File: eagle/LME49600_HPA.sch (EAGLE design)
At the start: 23 parts, among them IC1 OPA2134P, P1 POLYSWITCH, P2 POLYSWITCH

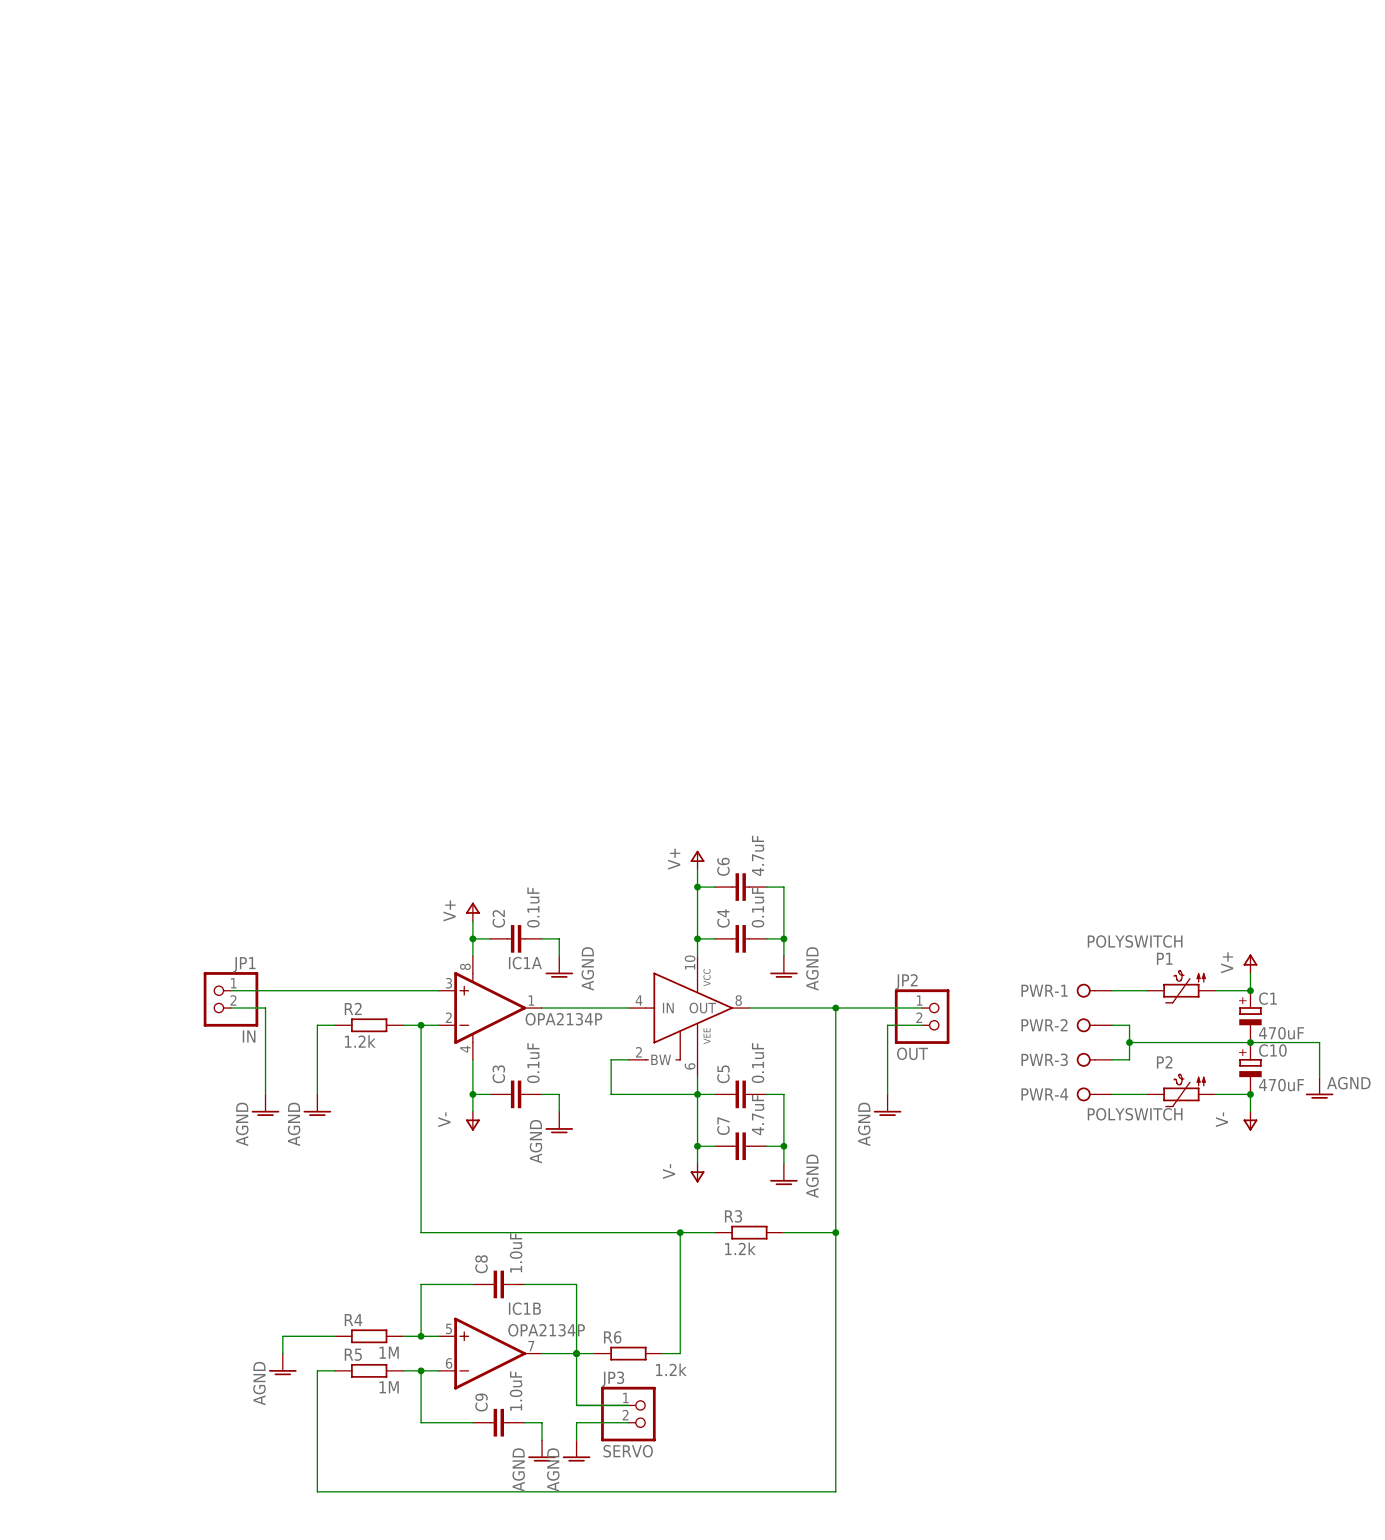
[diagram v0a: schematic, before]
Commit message: 2ch
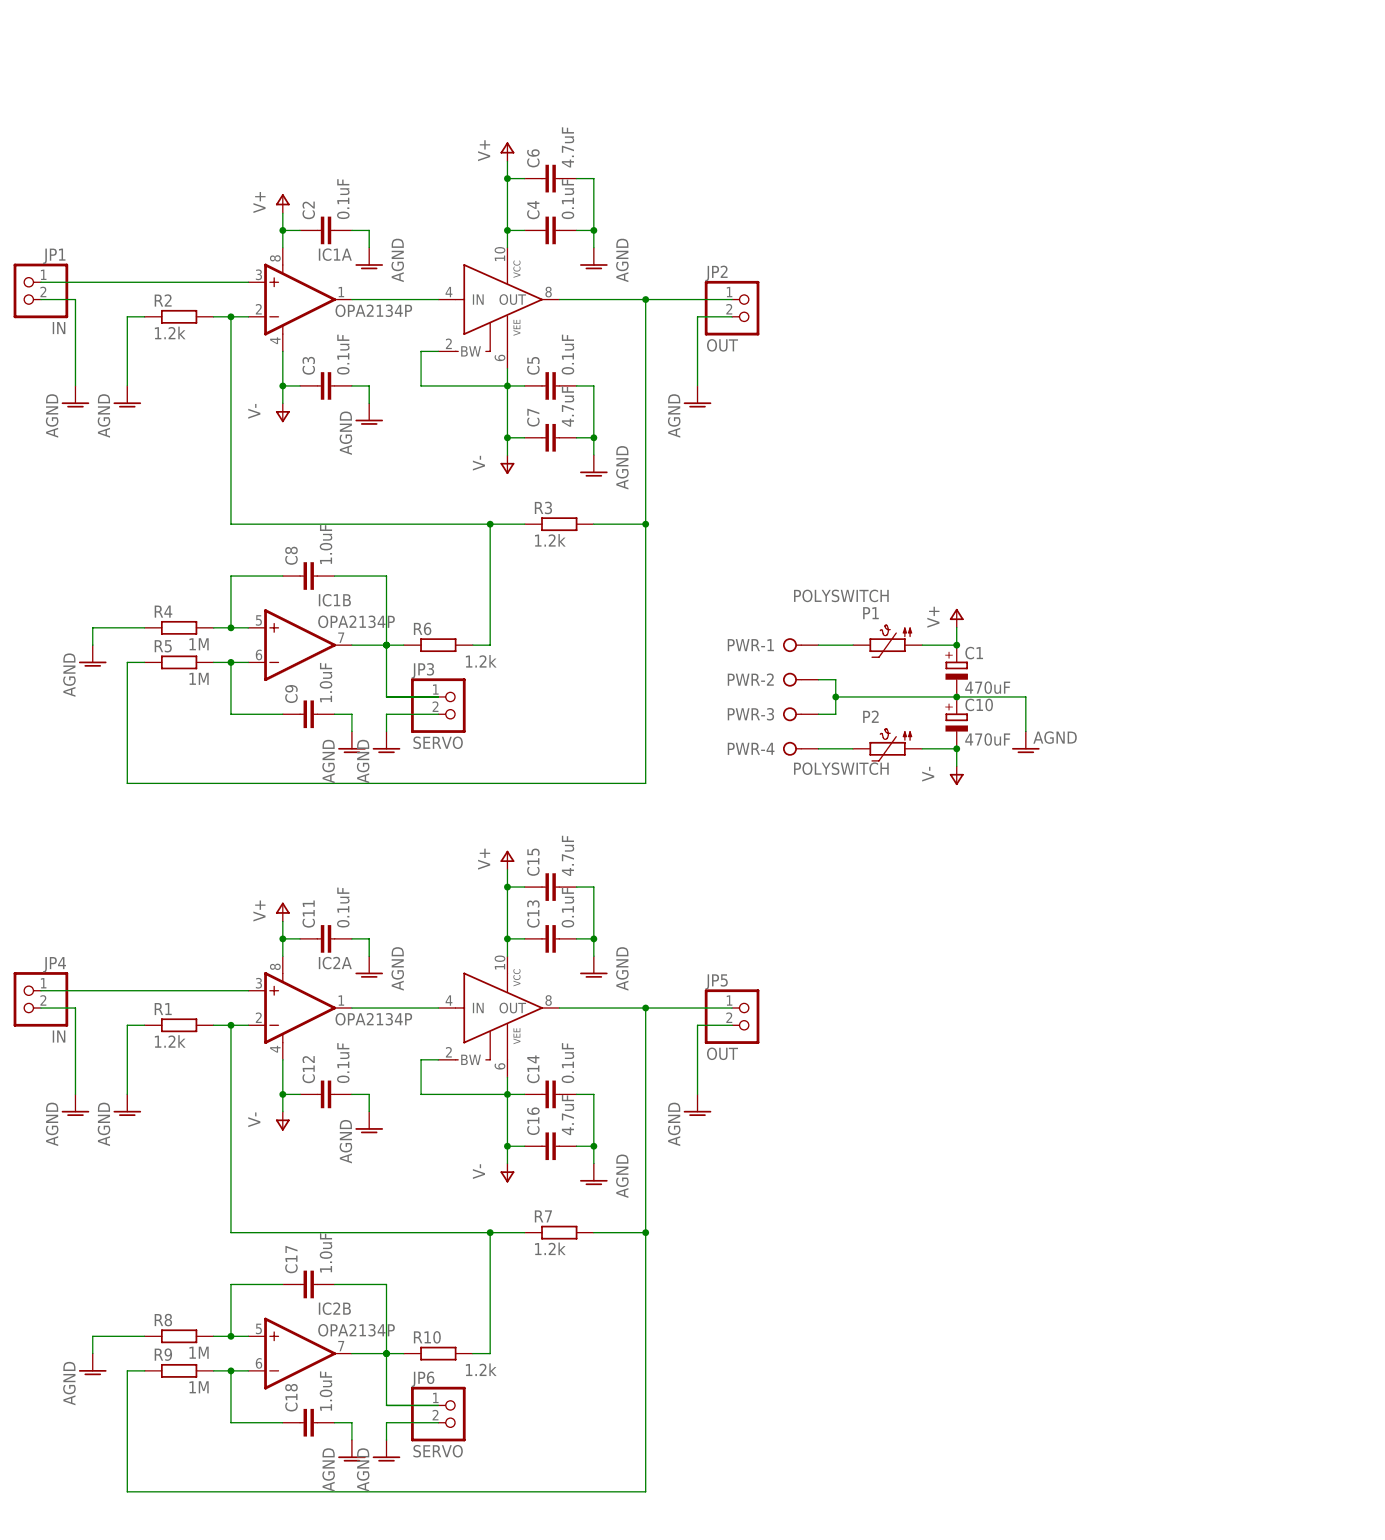
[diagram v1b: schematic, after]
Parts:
- added C11, C12, C13, C14: 0.1uF, rcl:C-EU075-042X103
- added C15, C16: 4.7uF, rcl:C-EU075-042X103
- added C17, C18: 1.0uF, rcl:C-EU050-050X075
- added IC2: OPA2134P, burr-brown:OPA2134P
- added JP4: IN, pinhead:PINHD-1X2
- added JP5: OUT, pinhead:PINHD-1X2
- added JP6: SERVO, pinhead:PINHD-1X2
- added R1, R10, R7: 1.2k, rcl:R-EU_0207/7
- added R8, R9: 1M, rcl:R-EU_0207/7
- added U$2: LME49600_BRD, mylib2:LME49600_BRD
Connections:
- new net N$10: C18.1, IC2B.-IN, R9.2
- new net N$12: C17.2, IC2B.OUT, JP6.1, R10.1
- new net N$13: JP5.1, R7.2, R9.1, U$2.OUT
- new net N$15: IC2A.+IN, JP4.1
- new net N$2: IC2A.-IN, R1.2, R10.2, R7.1
- new net N$4: IC2A.OUT, U$2.IN
- new net N$5: C17.1, IC2B.+IN, R8.2
- net AGND: now also C11.2, C12.2, C13.2, C14.2, C15.2, C16.2, C18.2, JP4.2, JP5.2, JP6.2, R1.1, R8.1
- net V+: now also C11.1, C13.1, C15.1, IC2A.V+, U$2.VCC
- net V-: now also C12.1, C14.1, C16.1, IC2A.V-, U$2.BW, U$2.VEE@1
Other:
- moved on the sheet: C1, C10, C2, C3, C4, C5, C6, C7, C8, C9, IC1A, IC1B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

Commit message: bug fix
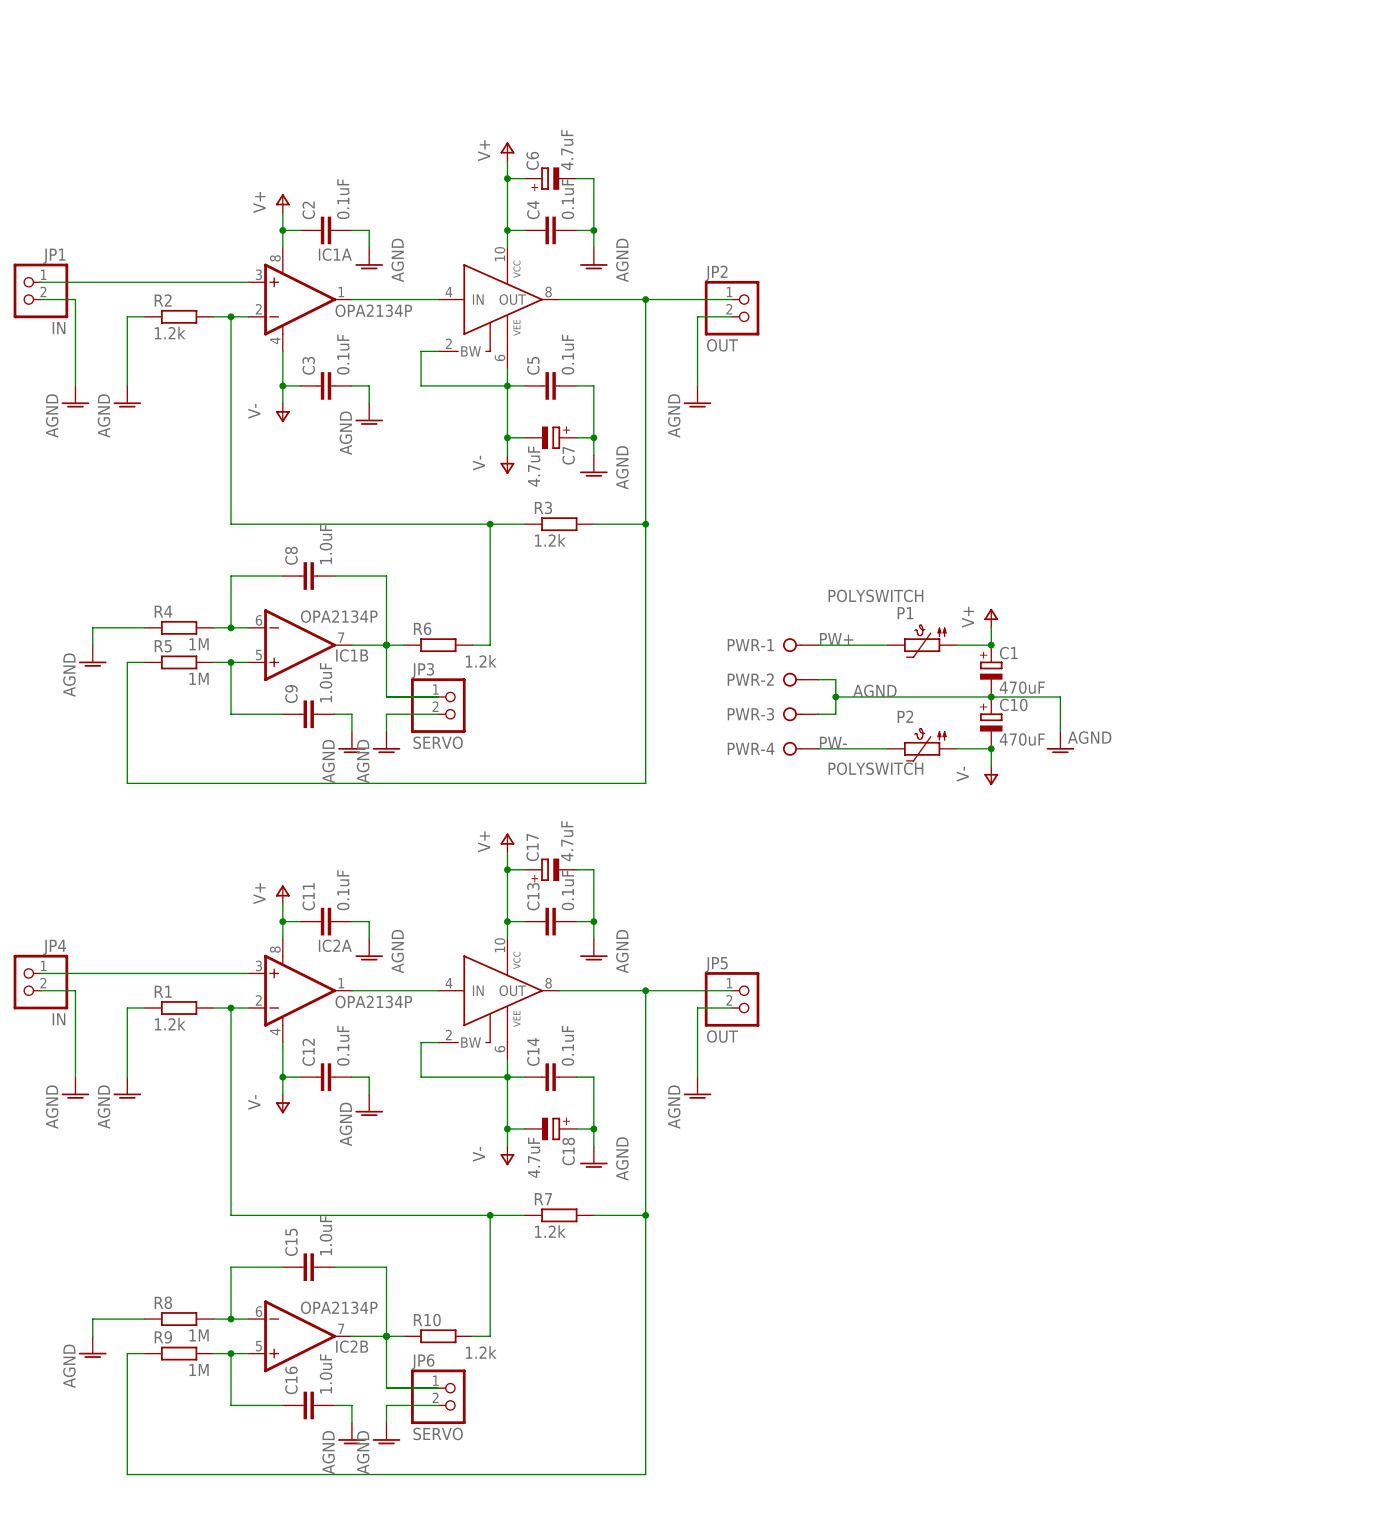
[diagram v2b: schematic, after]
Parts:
- C15, C16: value 4.7uF -> 1.0uF; device rcl:C-EU075-042X103 -> rcl:C-EU050-050X075
- C17, C18: value 1.0uF -> 4.7uF; device rcl:C-EU050-050X075 -> rcl:CPOL-EUE2-4
- C6, C7: device rcl:C-EU075-042X103 -> rcl:CPOL-EUE2-4
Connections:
- net N$9 renamed PW-
- net P1 renamed PW+
- removed net N$12 (its old number): C17.2, IC2B.OUT, JP6.1, R10.1
- new net N$9: C16.1, IC2B.+IN, R9.2
- net AGND: now also C17.-, C18.+, C6.-, C7.+; no longer C15.2, C18.2, C6.2, C7.2
- net N$10: now also C15.2, IC2B.OUT, JP6.1, R10.1; no longer C18.1, IC2B.-IN, R9.2
- net N$5: now also C15.1, IC2B.-IN; no longer C17.1, IC2B.+IN
- net N$6: now also IC1B.-IN; no longer IC1B.+IN
- net N$8: now also IC1B.+IN; no longer IC1B.-IN
- net V+: now also C17.+, C6.+; no longer C15.1, C6.1
- net V-: now also C18.-, C7.-; no longer C16.1, C7.1
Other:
- moved on the sheet: C1, C10, C11, C12, C13, C14, C15, C16, IC1B, IC2A, IC2B, JP4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

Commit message: bug fix
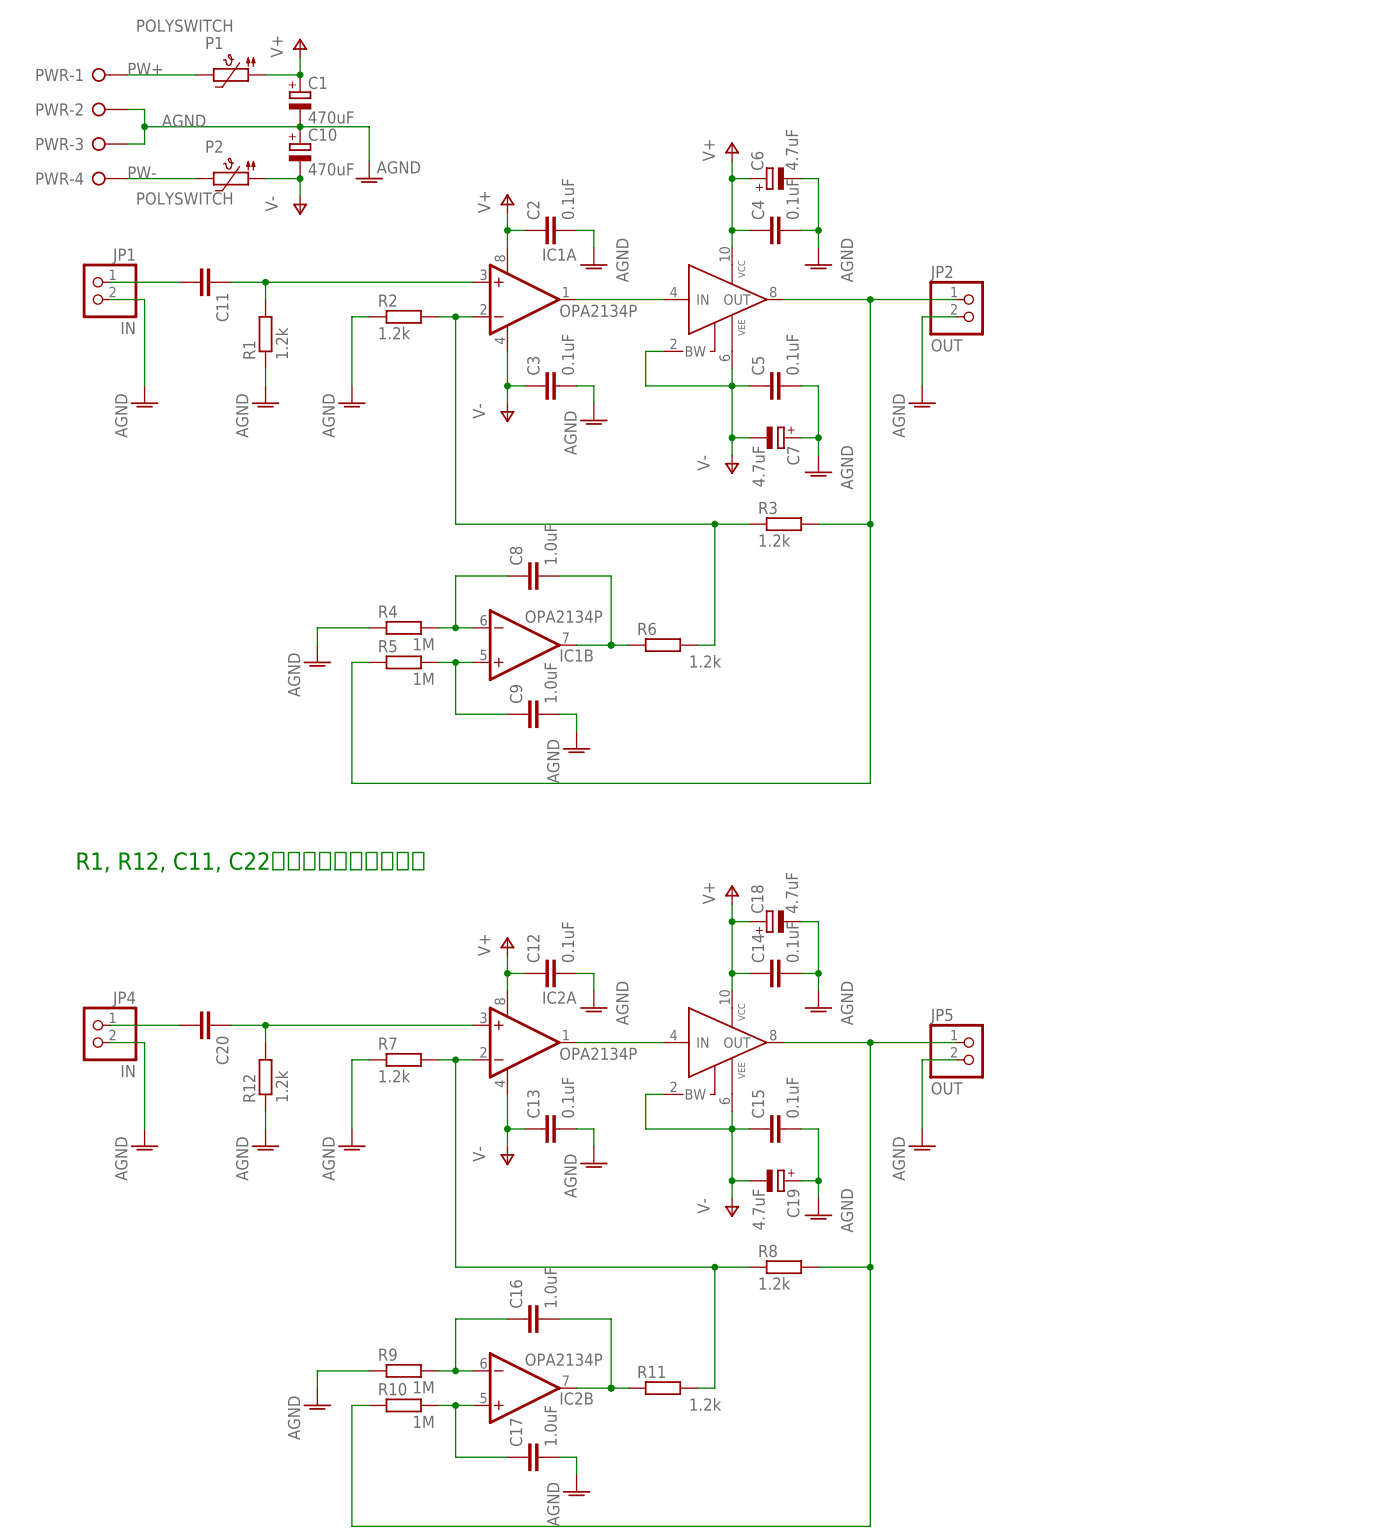
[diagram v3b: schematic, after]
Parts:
- removed JP3, JP6: SERVO, pinhead:PINHD-1X2
- added C19: 4.7uF, rcl:CPOL-EUE2-4
- added C20: (no value), rcl:C-EU050-055X075
- added R11, R12: 1.2k, rcl:R-EU_0207/7
- C11: value 0.1uF -> (none); device rcl:C-EU075-042X103 -> rcl:C-EU050-055X075
- C15: value 1.0uF -> 0.1uF; device rcl:C-EU050-050X075 -> rcl:C-EU075-042X103
- C17: value 4.7uF -> 1.0uF; device rcl:CPOL-EUE2-4 -> rcl:C-EU050-050X075
- R10: value 1.2k -> 1M
- R8: value 1M -> 1.2k
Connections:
- removed net N$5 (its old number): C15.1, IC2B.-IN, R8.2
- new net N$15: C20.2, JP4.1
- new net N$16: C20.1, IC2A.+IN, R12.2
- new net N$4: IC2A.-IN, R11.2, R7.2, R8.1
- net AGND: now also C15.2, C17.2, C18.-, C19.+, R12.1, R7.1, R9.1; no longer C11.2, C16.2, C17.-, C18.+, JP3.2, JP6.2, R8.1
- net N$1: now also C11.2; no longer IC1A.+IN
- net N$10: now also C17.1, IC2B.+IN, R10.2; no longer C15.2, IC2B.OUT, JP6.1, R10.1
- net N$11: no longer JP3.1
- net N$12: now also C16.2, IC2B.OUT, R11.1; no longer JP5.1, R7.2, R9.1, U$2.OUT
- net N$13: now also JP5.1, R10.1, R8.2, U$2.OUT; no longer IC2A.+IN, JP4.1
- net N$2: now also C11.1, IC1A.+IN; no longer IC2A.-IN, R10.2, R7.1
- net N$9: now also IC2B.-IN; no longer IC2B.+IN
- net V+: now also C12.1, C14.1, C18.+; no longer C11.1, C13.1, C17.+
- net V-: now also C13.1, C15.1, C19.-; no longer C12.1, C14.1, C18.-
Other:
- note added: "R1, R12, C11, C22はピンソケットで実装"
- moved on the sheet: C1, C10, C11, C12, C13, C14, C15, C16, C18, C2, C3, C4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
